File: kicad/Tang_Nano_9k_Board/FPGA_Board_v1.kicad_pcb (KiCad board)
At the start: 2 copper layers, 11 parts, among them U3 TBD62083AFG, U5 TBD62783A

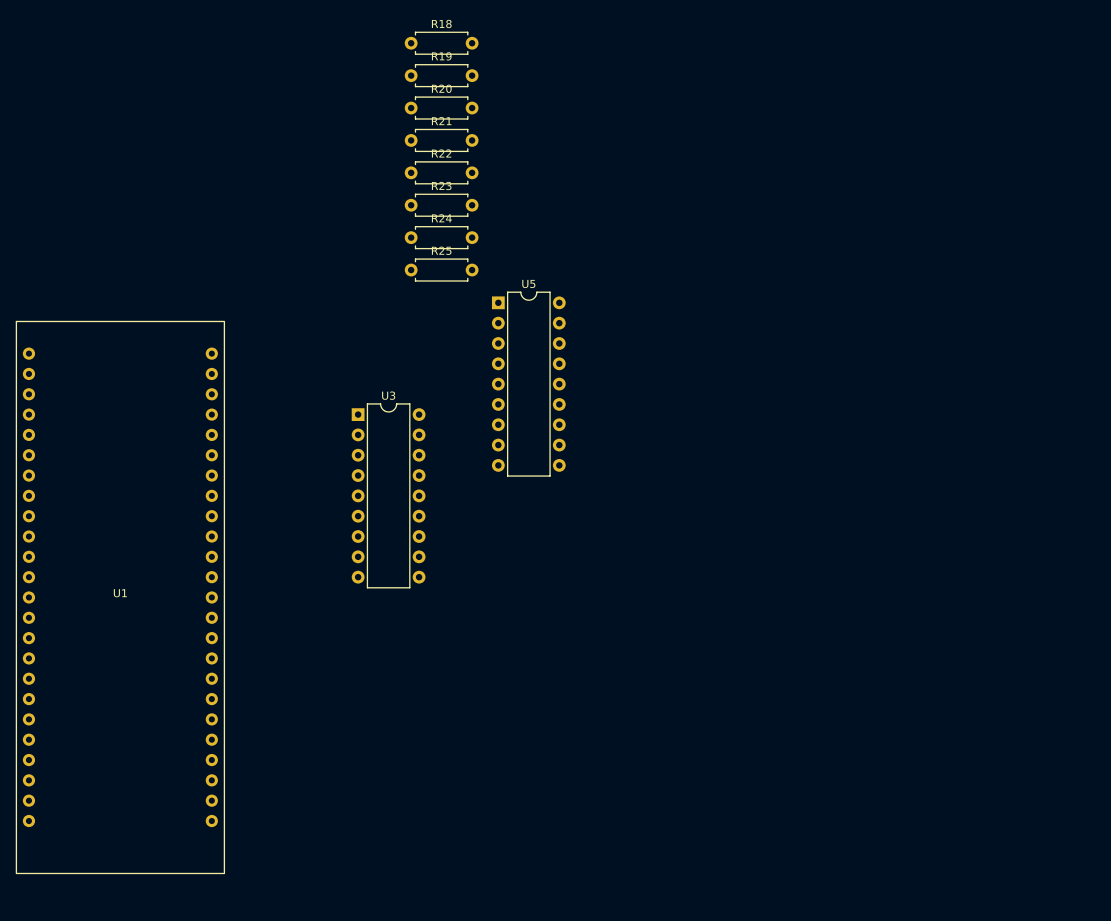
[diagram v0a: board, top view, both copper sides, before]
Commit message: making pcb board
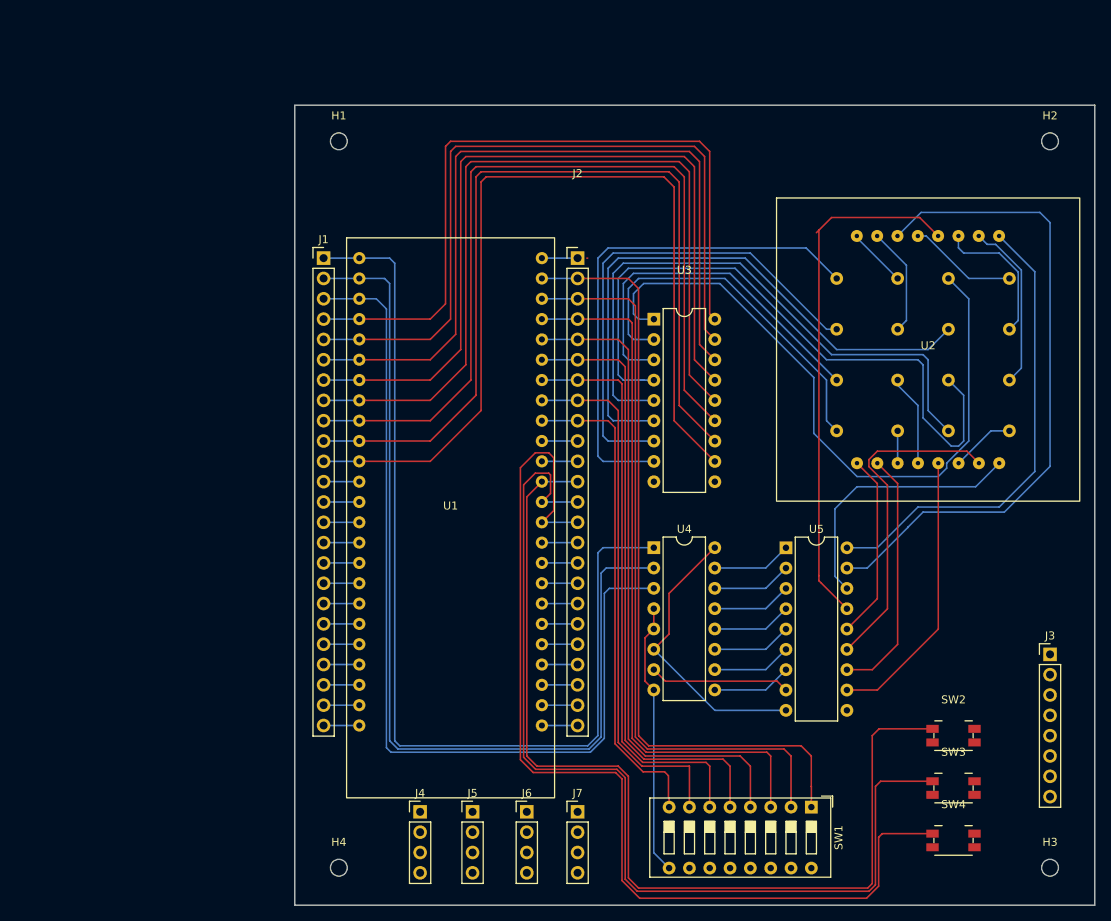
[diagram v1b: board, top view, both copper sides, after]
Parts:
- added H1: MountingHole, MountingHole:MountingHole_2.1mm, F.Cu at (103.5, 56.5)
- added H2: MountingHole, MountingHole:MountingHole_2.1mm, F.Cu at (192.4, 56.5)
- added H3: MountingHole, MountingHole:MountingHole_2.1mm, F.Cu at (192.4, 147.3)
- added H4: MountingHole, MountingHole:MountingHole_2.1mm, F.Cu at (103.5, 147.3)
- added J1: Conn_01x24, Connector_PinHeader_2.54mm:PinHeader_1x24_P2.54mm_Vertical, F.Cu at (101.6, 71.1)
- added J2: Conn_01x24, Connector_PinHeader_2.54mm:PinHeader_1x24_P2.54mm_Vertical, F.Cu at (133.3, 71.1)
- added J3: Conn_01x08, Connector_PinHeader_2.54mm:PinHeader_1x08_P2.54mm_Vertical, F.Cu at (192.4, 120.7)
- added J4: Conn_01x04, Connector_PinHeader_2.54mm:PinHeader_1x04_P2.54mm_Vertical, F.Cu at (113.7, 140.3)
- added J5: Conn_01x04, Connector_PinHeader_2.54mm:PinHeader_1x04_P2.54mm_Vertical, F.Cu at (120.2, 140.3)
- added J6: Conn_01x04, Connector_PinHeader_2.54mm:PinHeader_1x04_P2.54mm_Vertical, F.Cu at (127.0, 140.3)
- added J7: Conn_01x04, Connector_PinHeader_2.54mm:PinHeader_1x04_P2.54mm_Vertical, F.Cu at (133.3, 140.3)
- added SW1: SW_DIP_x08, Button_Switch_THT:SW_DIP_SPSTx08_Slide_9.78x22.5mm_W7.62mm_P2.54mm, F.Cu at (162.6, 139.7)
- added SW2: SW_Push, Button_Switch_SMD:Panasonic_EVQPUJ_EVQPUA, F.Cu at (180.3, 130.8)
- added SW3: SW_Push, Button_Switch_SMD:Panasonic_EVQPUJ_EVQPUA, F.Cu at (180.3, 137.4)
- added SW4: SW_Push, Button_Switch_SMD:Panasonic_EVQPUJ_EVQPUA, F.Cu at (180.3, 143.9)
- added U2: ~, BFP_footprints:OSL641501-BX, F.Cu at (177.2, 82.5)
- added U4: 74HC138, Package_DIP:CERDIP-16_W7.62mm_SideBrazed, F.Cu at (142.9, 107.3)
- R18, R19, R20, R21, R22, R23, R24, R25: value 600 -> 750; moved to B.Cu
- U1: footprint BFP:Tang_Nano_9K -> BFP_footprints:Tang_Nano_9K
- moved R22 81.4 mm to (187.3, 92.7), turned to 180 degrees
- moved R21 80.6 mm to (187.3, 86.4), turned to 180 degrees
- moved R18 80.4 mm to (187.3, 73.7), turned to 180 degrees
- moved R23 76.4 mm to (187.3, 80.0), turned to 180 degrees
- moved R19 75.3 mm to (173.4, 92.7), turned to 180 degrees
- moved R20 69.7 mm to (173.4, 86.4), turned to 180 degrees
- moved R24 61.9 mm to (173.4, 80.0), turned to 180 degrees
- moved R25 60.8 mm to (173.4, 73.7), turned to 180 degrees
- moved U5 47.2 mm to (159.4, 107.3)
- moved U1 42.5 mm to (117.5, 103.6)
- moved U3 38.8 mm to (142.9, 78.8)
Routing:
- net Net-(J2-Pin_14): track 0.00 -> 127.9 mm
- net Net-(J1-Pin_1): track 0.00 -> 125.2 mm
- net Net-(J2-Pin_13): track 0.00 -> 124.8 mm
- net Net-(J2-Pin_12): track 0.00 -> 123.6 mm
- net Net-(J1-Pin_2): track 0.00 -> 120.5 mm
- net Net-(J1-Pin_3): track 0.00 -> 116.0 mm
- net /C8: track 0.00 -> 112.2 mm
- net /C7: track 0.00 -> 109.2 mm
- net /C6: track 0.00 -> 106.1 mm
- net /C5: track 0.00 -> 103.0 mm
- net /C4: track 0.00 -> 100.0 mm
- net Net-(J2-Pin_2): track 0.00 -> 97.5 mm
- net /C3: track 0.00 -> 96.9 mm
- net /C2: track 0.00 -> 93.8 mm
- net Net-(J2-Pin_3): track 0.00 -> 92.8 mm
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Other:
- board outline added: 100 x 100 mm
